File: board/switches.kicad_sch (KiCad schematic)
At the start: 3 parts, among them Q1 BUK7880-55A, U1 LTC7001

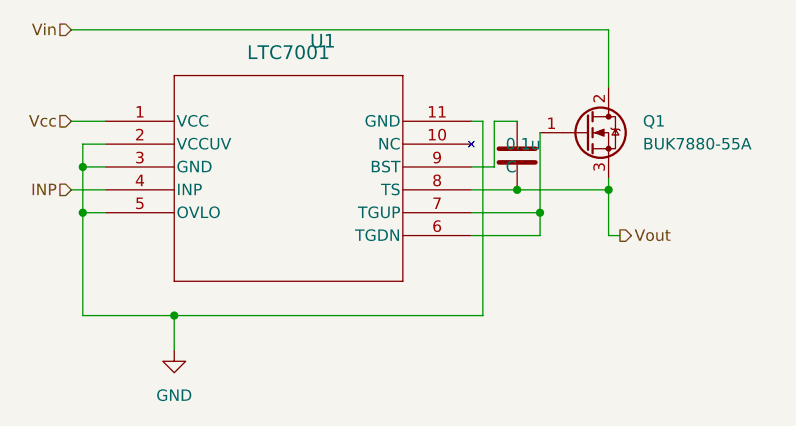
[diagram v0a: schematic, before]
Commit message: Changed Flags
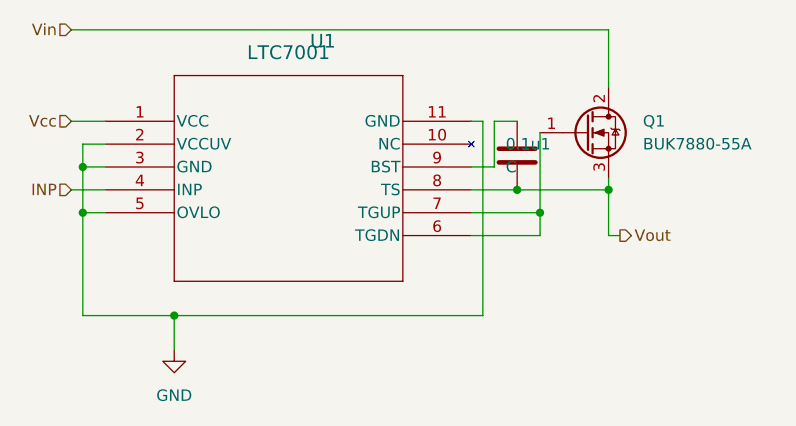
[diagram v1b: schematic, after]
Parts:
- renumbered 0.1u to 0.1u1
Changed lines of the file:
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@@
 		(on_board yes)
 		(dnp no)
-		(property "Reference" "0.1u"
+		(property "Reference" "0.1u1"
 			(at 140.97 77.47 0)
 			(effects
@@
 			(project ""
 				(path "/7eaa639d-7062-45e7-be05-1c2855431307/d051b168-830a-4a55-b5cd-142fa18015a1"
-					(reference "0.1u")
+					(reference "0.1u1")
 					(unit 1)
 				)
